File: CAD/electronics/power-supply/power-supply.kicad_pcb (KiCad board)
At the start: 2 copper layers, 67.9 x 54 mm, 26 parts, among them J1 Batterie, J2 12V, J3 5V servo, U1 LM7805_TO220, U3 LM741, U6 LM2576T-5

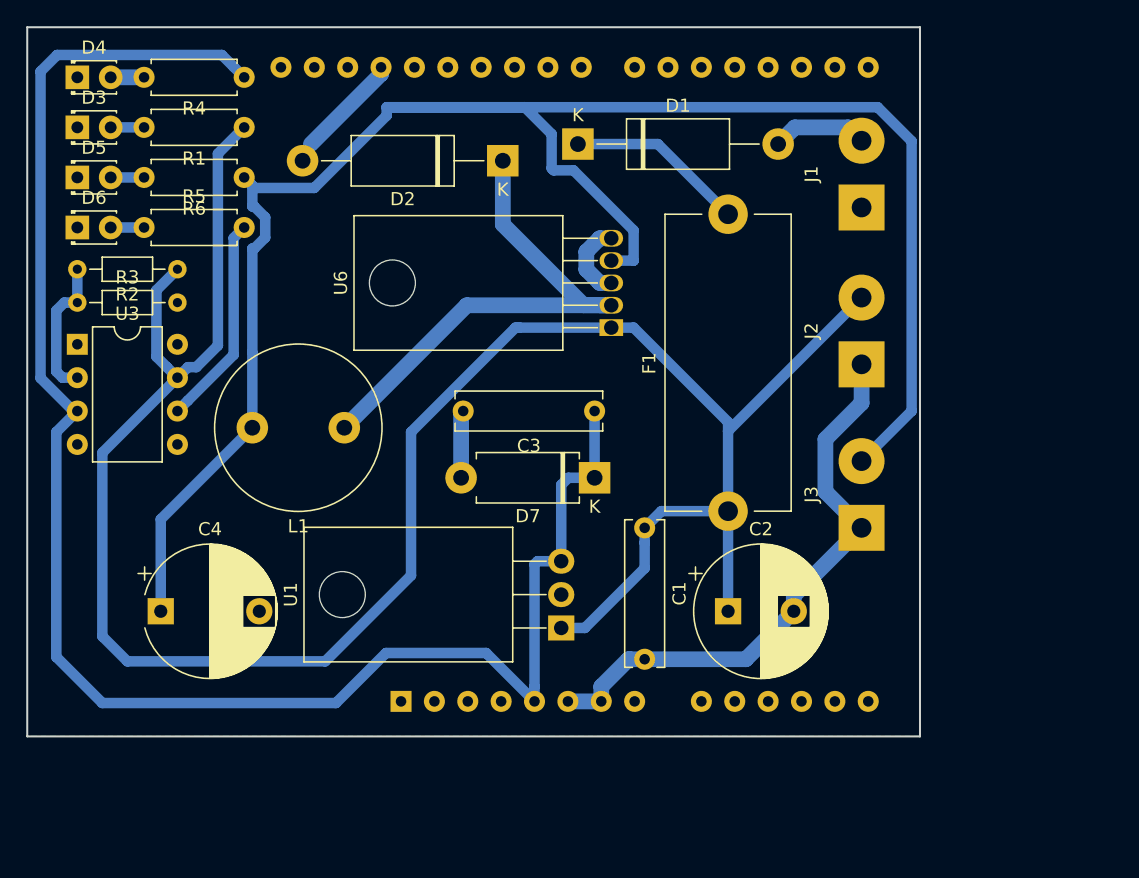
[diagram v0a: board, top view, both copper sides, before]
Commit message: Electronics sent to manufacturer
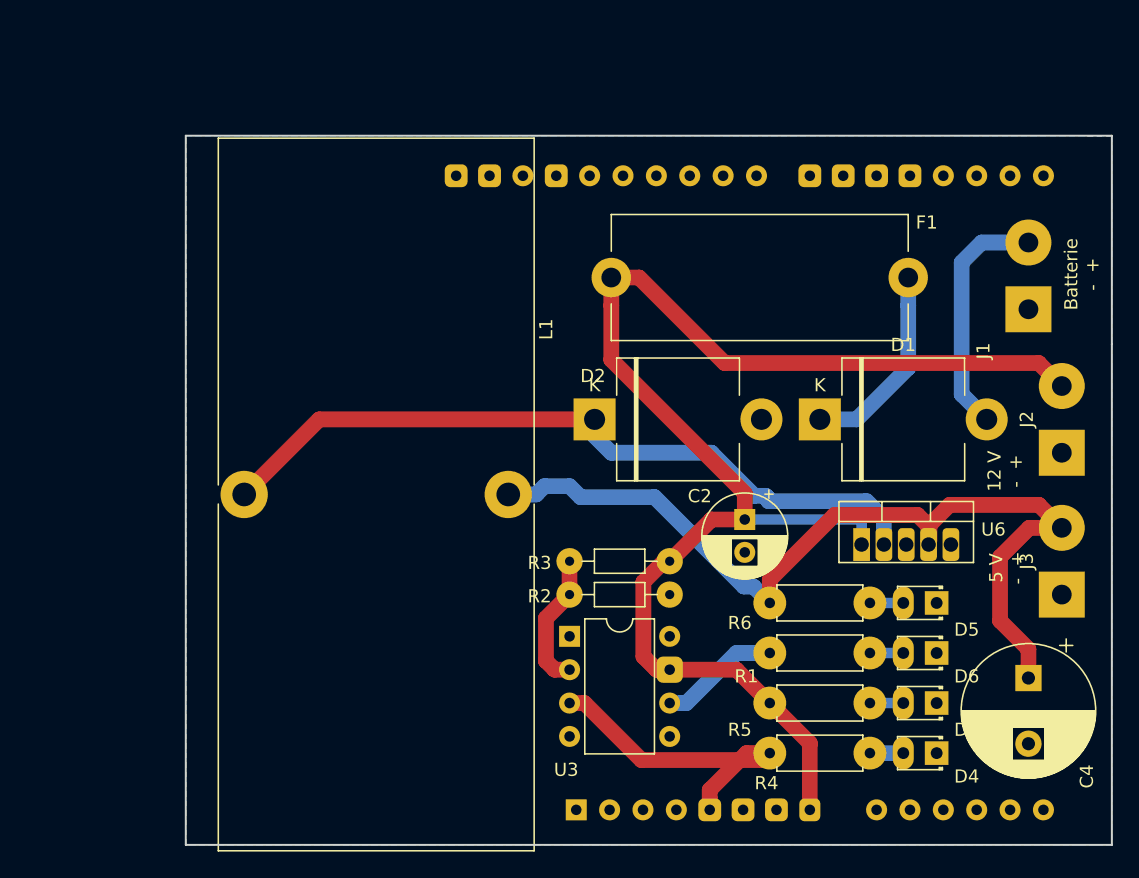
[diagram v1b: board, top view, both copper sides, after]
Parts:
- removed C1: 330n, Capacitor_THT:C_Rect_L11.0mm_W2.8mm_P10.00mm_MKT
- removed C3: 100n, Capacitor_THT:C_Rect_L11.0mm_W2.8mm_P10.00mm_MKT
- removed D7: 6V Zener, Diode_THT:D_DO-15_P10.16mm_Horizontal
- removed U1: LM7805_TO220, Package_TO_SOT_THT:TO-220-3_Horizontal_TabDown
- C2: footprint Capacitor_THT:CP_Radial_D10.0mm_P5.00mm -> Capacitor_THT:CP_Radial_D6.3mm_P2.50mm
- C4: footprint Capacitor_THT:CP_Radial_D10.0mm_P7.50mm -> Capacitor_THT:CP_Radial_D10.0mm_P5.00mm
- D1, D2: footprint Diode_THT:D_DO-15_P15.24mm_Horizontal -> Diode_THT:D_P600_R-6_P12.70mm_Horizontal
- L1: footprint Inductor_THT:L_Radial_D12.5mm_P7.00mm_Fastron_09HCP -> Inductor_THT:L_Toroid_Vertical_L54.0mm_W23.8mm_P20.10mm_Bourns_5700
- U6: footprint Package_TO_SOT_THT:TO-220-5_Horizontal_TabDown -> Package_TO_SOT_THT:TO-220-5_Vertical
- moved D4 83.2 mm to (100.3, 79.8), turned to 180 degrees
- moved D3 78.7 mm to (100.3, 75.9), turned to 180 degrees
- moved D5 73.0 mm to (100.3, 68.3), turned to 180 degrees
- moved D6 73.0 mm to (100.3, 72.1), turned to 180 degrees
- moved C4 66.2 mm to (107.3, 74.0), turned to 270 degrees
- moved R4 65.2 mm to (87.6, 79.8), turned to 0 degrees
- moved R5 64.0 mm to (95.2, 72.1), turned to 180 degrees
- moved R1 59.3 mm to (87.6, 75.9), turned to 0 degrees
- moved R6 51.5 mm to (87.6, 68.3), turned to 0 degrees
- moved R2 43.6 mm to (80.0, 65.2)
- moved R3 43.6 mm to (72.4, 67.7)
- moved U3 43.6 mm to (72.4, 70.9)
- moved D1 27.9 mm to (91.4, 54.4)
- moved U6 25.2 mm to (94.6, 63.9), turned to 0 degrees
- moved D2 20.9 mm to (74.3, 54.4), turned to 0 degrees
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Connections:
- A1 pad 8: Net-(A1-Pad8) -> 12V
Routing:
- net 5V_logic: track 130.4 -> 24.8 mm
- net 5V_servo: track 146.4 -> 70.2 mm
- net GND: track 63.1 -> 0.00 mm
- net 12V: track 168.4 -> 107.1 mm
- net Net-(D2-Pad1): track 40.7 -> 57.0 mm
- net Net-(D1-Pad2): track 7.30 -> 18.4 mm
- net Net-(R5-Pad2): track 16.1 -> 9.20 mm
- net Net-(D1-Pad1): track 13.6 -> 15.2 mm
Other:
- board size 67.9 x 54 mm -> 70.5 x 54 mm
- net class Default: trace_width 0.8 -> 1.2
- board text added: "12 V - +"
- board text added: "5 V - +"
- board text added: "Batterie - +"
